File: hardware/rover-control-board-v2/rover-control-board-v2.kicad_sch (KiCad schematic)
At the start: 36 parts, among them J1 M6 Terminal, J10 CAN3, J2 M6 Terminal, J3 Contactor, J4 XT90_REG_OUT, J5 XT90_REG_RET, J6 OUT, J7 RET, J8 CAN1, J9 CAN2, Q5 MCACD8D5N06YL-TP

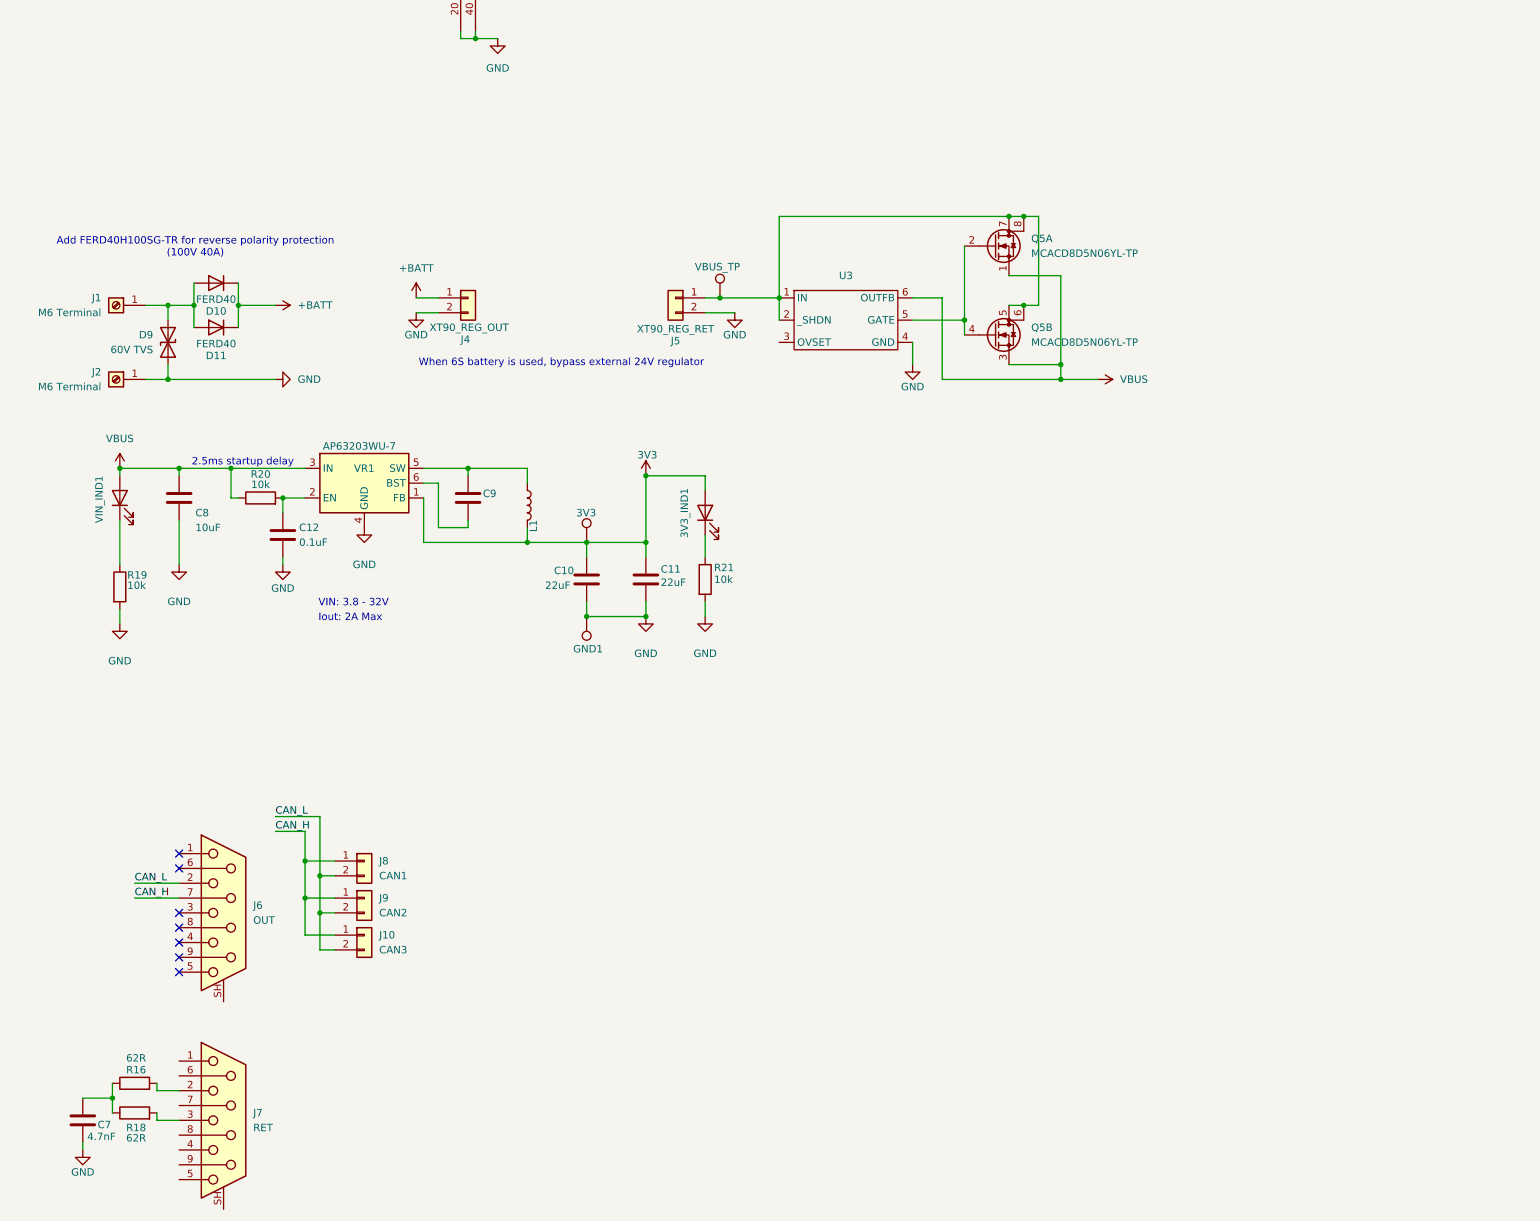
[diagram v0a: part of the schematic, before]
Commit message: Further protections
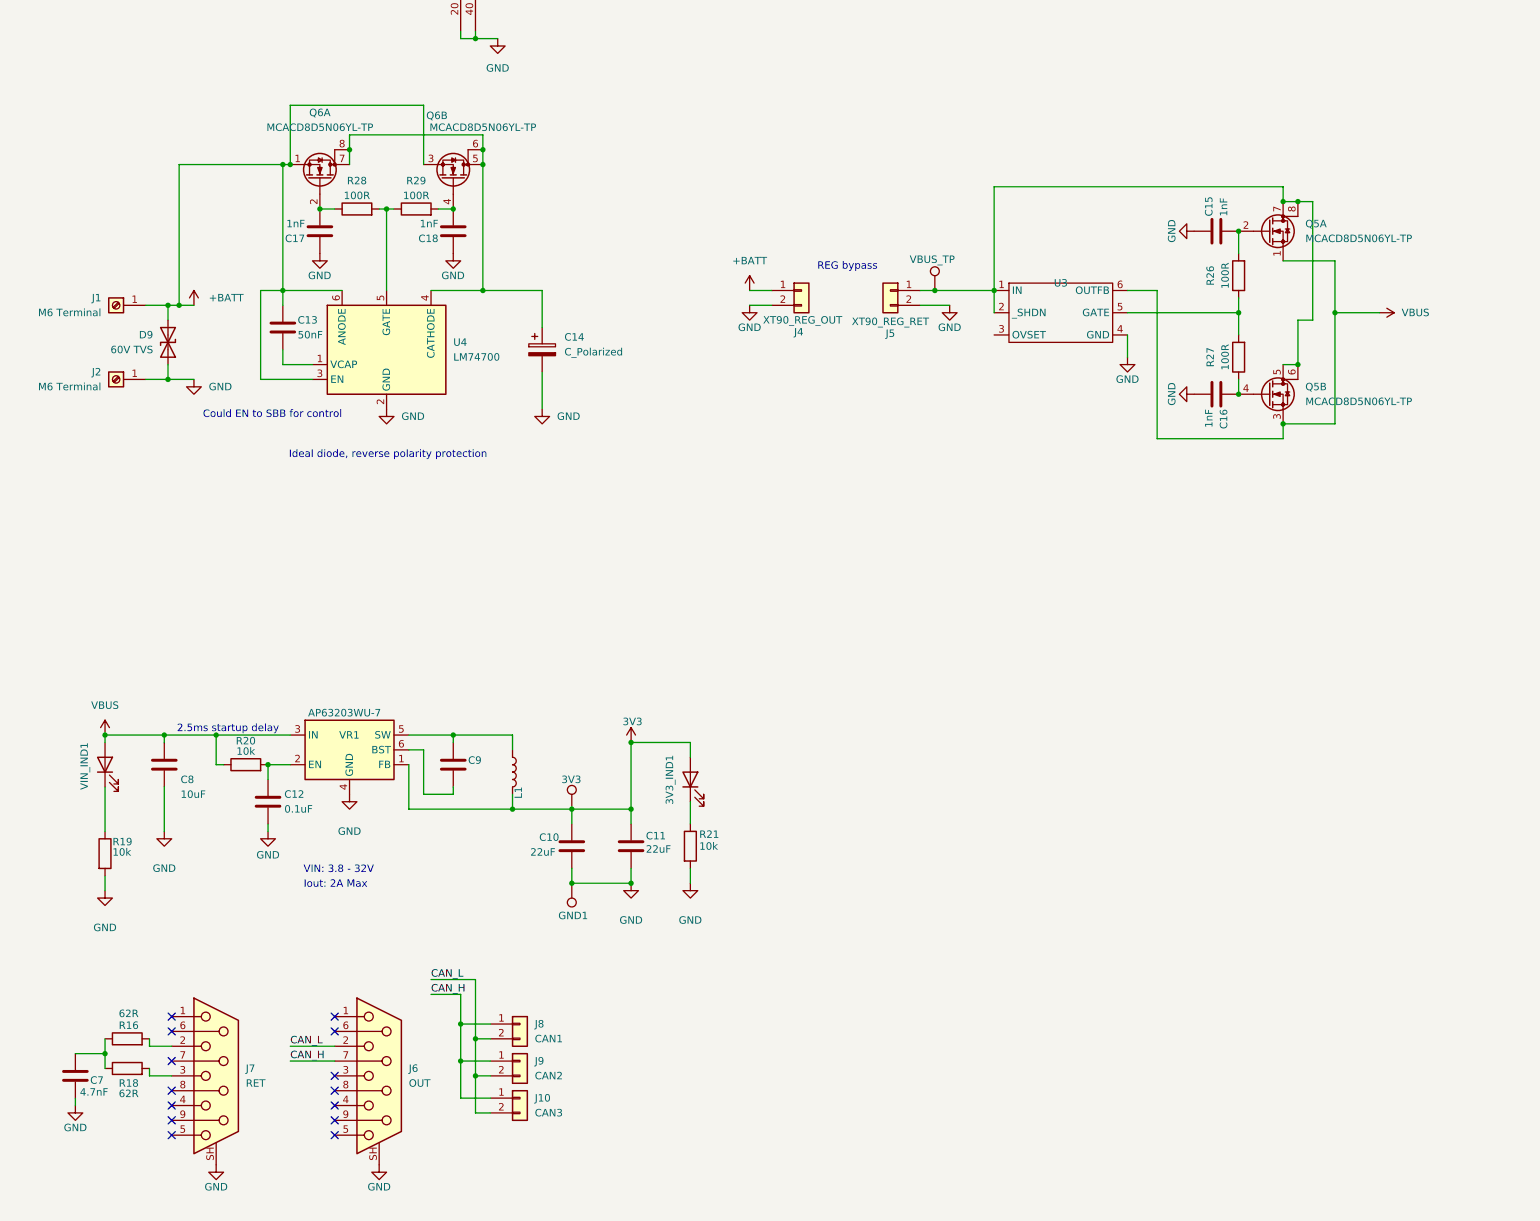
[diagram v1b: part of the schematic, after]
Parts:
- removed D10, D11: FERD40, Package_TO_SOT_SMD:TO-263-2_TabPin1, symbol Device:D
- added C13: 50nF, symbol Device:C
- added C14: C_Polarized, symbol Device:C_Polarized
- added C15, C16, C17, C18: 1nF, symbol Device:C
- added Q6: MCACD8D5N06YL-TP, symbol Transistor_FET:Q_Dual_NMOS_S1G1S2G2D2D2D1D1
- added R26, R27, R28, R29: 100R, symbol Device:R
- added U4: LM74700, Package_TO_SOT_SMD:SOT-23-6, symbol Power_Management:LM74700
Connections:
- net +BATT: now also D9.2 (A2), J1.1 (Pin_1), C13.1, Q6.1 (S), Q6.3 (S), U4.3 (EN), U4.6 (ANODE)
- net GND: now also J6.SH (PAD), J7.SH (PAD), C14.2, C15.1, C16.2, C17.1, C18.1, U4.2 (GND)
- new net: C18.2, Q6.4 (G), R29.2
- new net: C14.1, Q6.5 (D), Q6.6 (D), Q6.7 (D), Q6.8 (D), U4.4 (CATHODE)
- new net: C17.2, Q6.2 (G), R28.1
- new net: R28.2, R29.1, U4.5 (GATE)
- new net: C13.2, U4.1 (VCAP)
- new net: C16.1, Q5.4 (G), R27.1
- new net: R26.1, R27.2, U3.5 (GATE)
- new net: C15.2, Q5.2 (G), R26.2
- no-connect marks 8 -> 15
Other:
- note added: "Could EN to SBB for control"
- note added: "Ideal diode, reverse polarity protection"
- note added: "REG bypass"
- note removed: "Add FERD40H100SG-TR for reverse polarity protection (100V 40A)"
- note removed: "When 6S battery is used, bypass external 24V regulator"
- moved on the sheet: 3V3, 3V3_IND1, C10, C11, C12, C7, C8, C9, GND1, J10, J4, J5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
